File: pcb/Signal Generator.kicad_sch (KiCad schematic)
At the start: 6 parts, among them J1 AudioJack3, J2 Conn_02x02_Odd_Even, J3 Screw_Terminal_01x04, J4 MEM2080-00-128-00-A

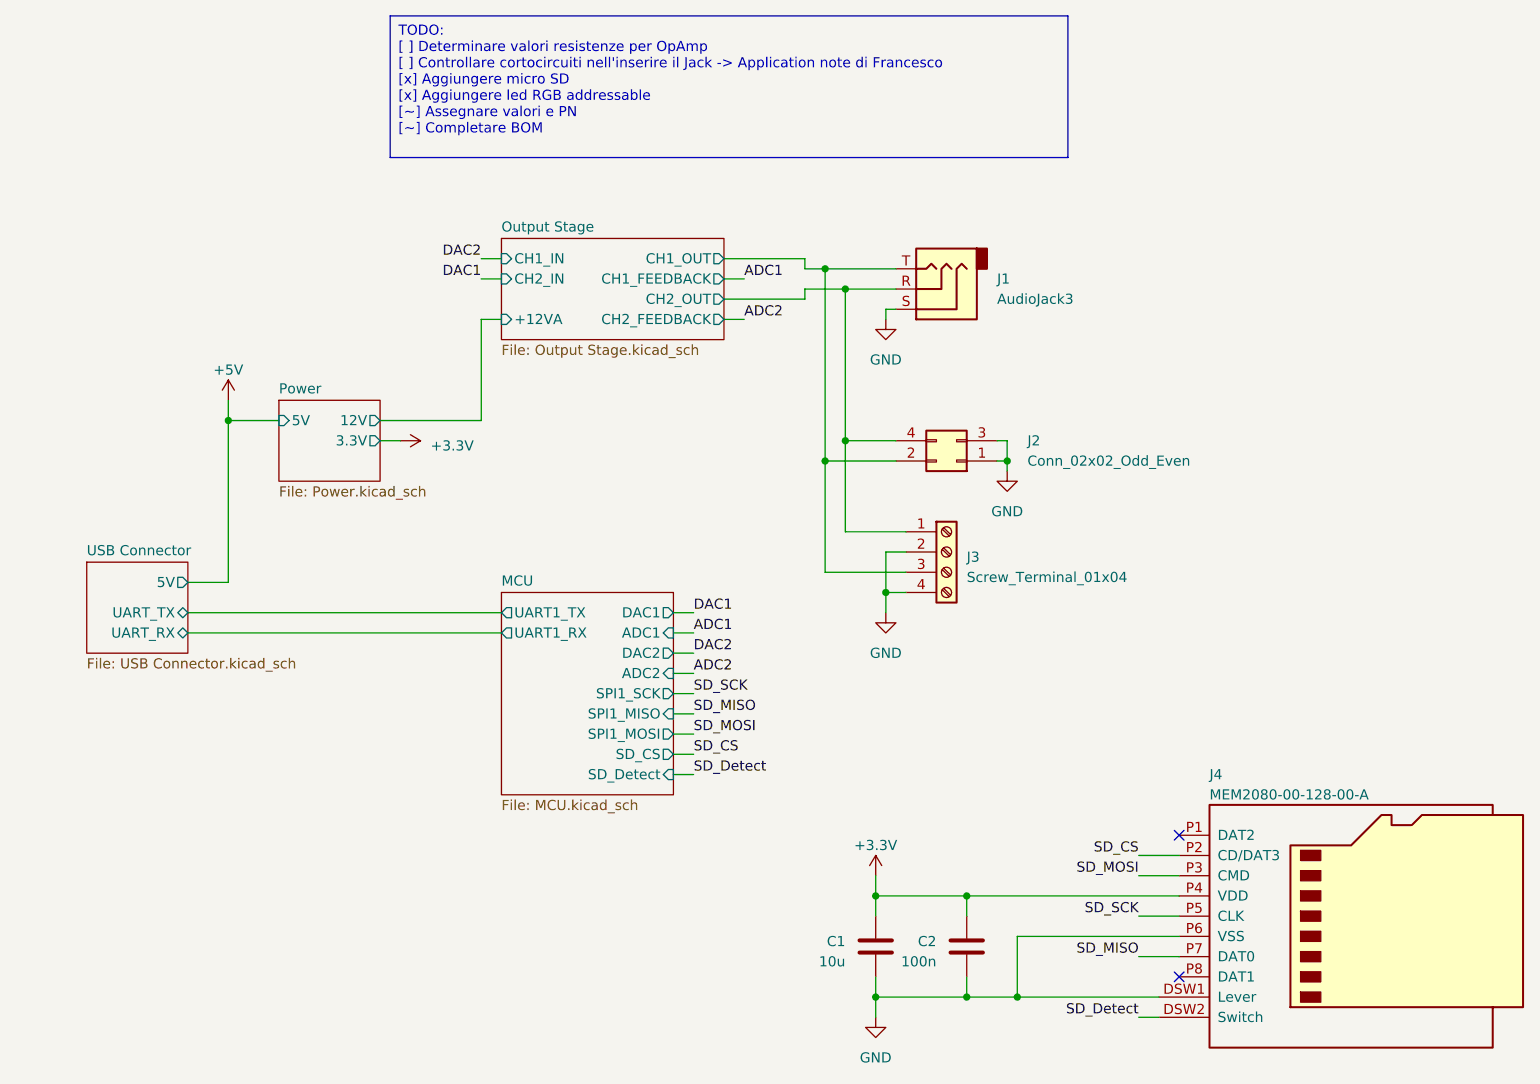
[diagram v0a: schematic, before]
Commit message: Completed schematic and tried some simulations
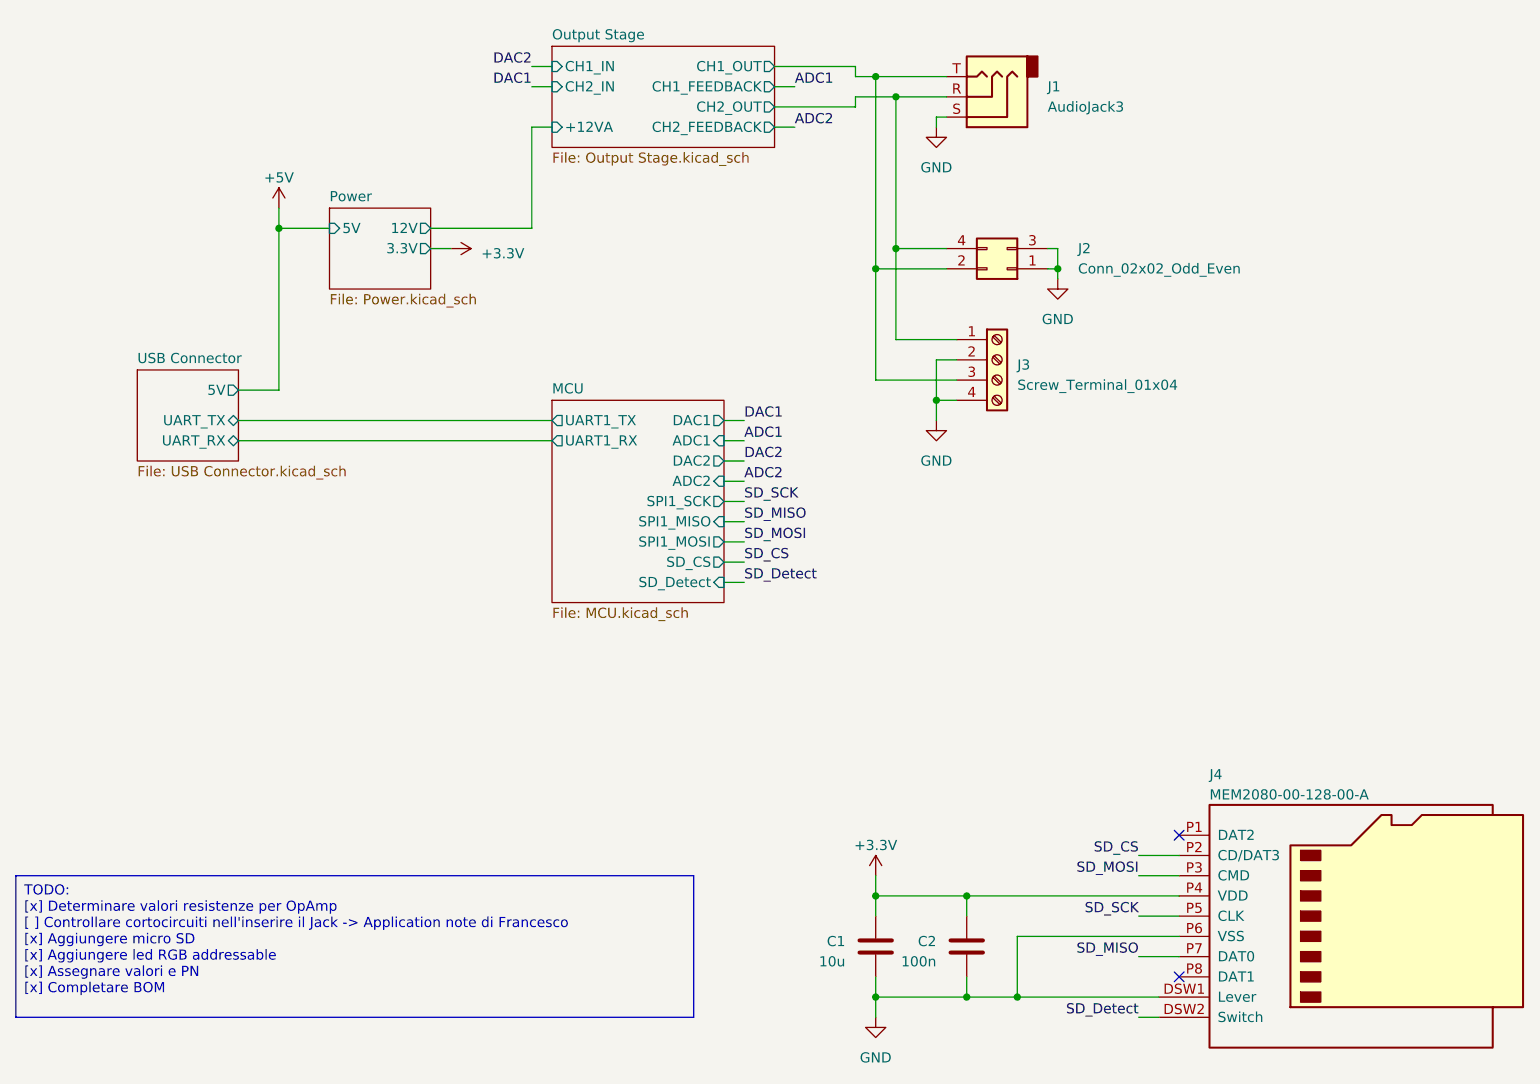
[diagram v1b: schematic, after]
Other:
- moved on the sheet: J1, J2, J3
